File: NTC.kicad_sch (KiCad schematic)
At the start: 16 parts, among them U3 LM1117GS-3.3, U4 LMV7219M5, U5 ADuM1200AR

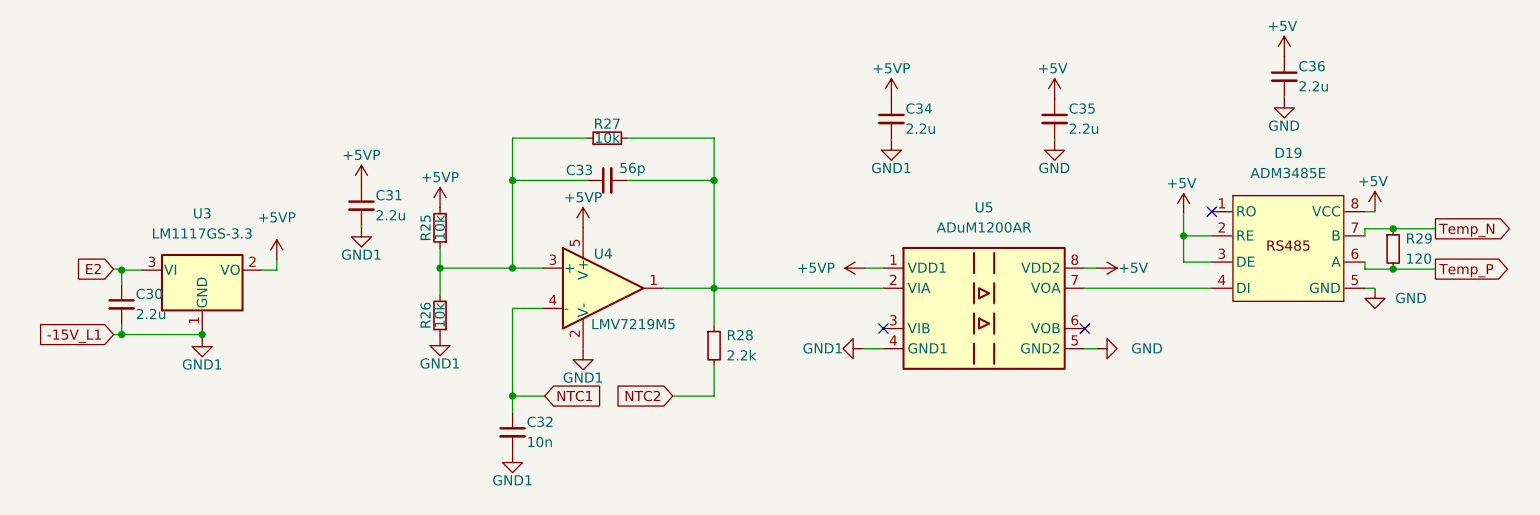
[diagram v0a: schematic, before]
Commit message: Развел все дорожки
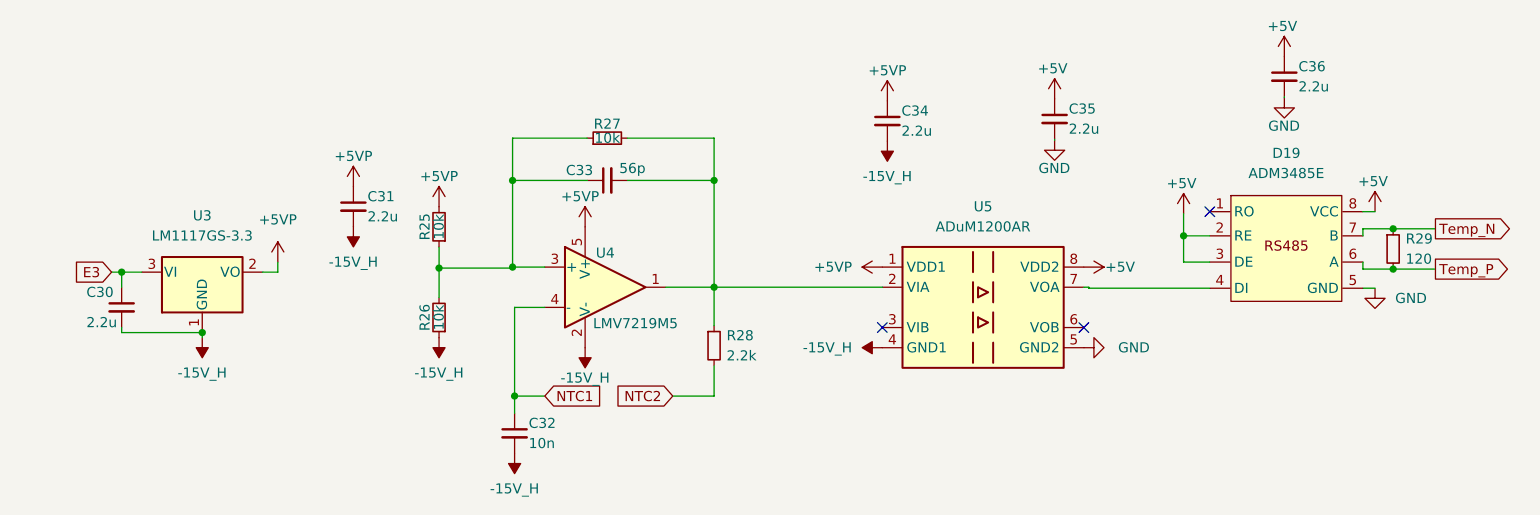
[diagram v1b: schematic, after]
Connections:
- net E2 renamed E3
- net GND1 renamed -15V_H
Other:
- moved on the sheet: C31, C34
